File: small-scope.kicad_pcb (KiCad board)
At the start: 2 copper layers, 35.6 x 53.3 mm, 41 parts, among them P1 BNC, P2 AREF, SW1 STAT DIS, U1 LM324N

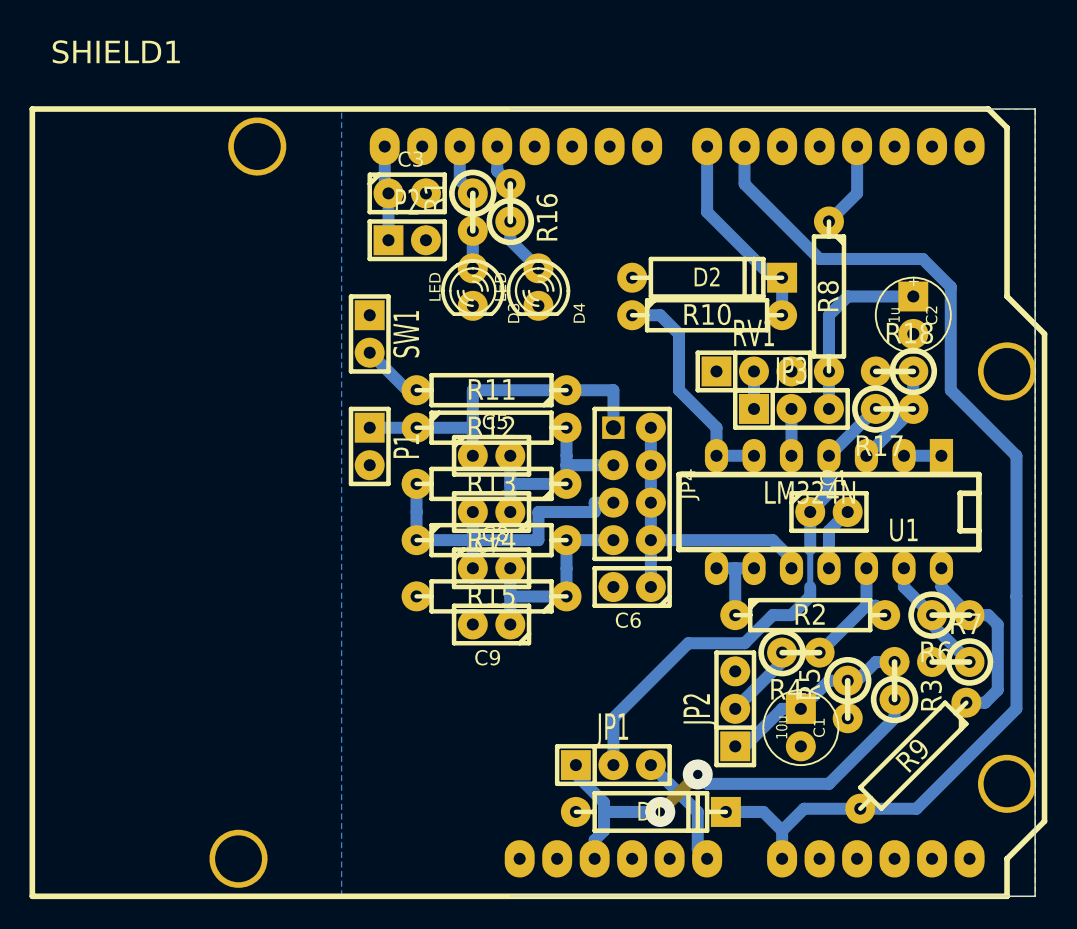
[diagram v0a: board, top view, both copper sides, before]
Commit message: routing done
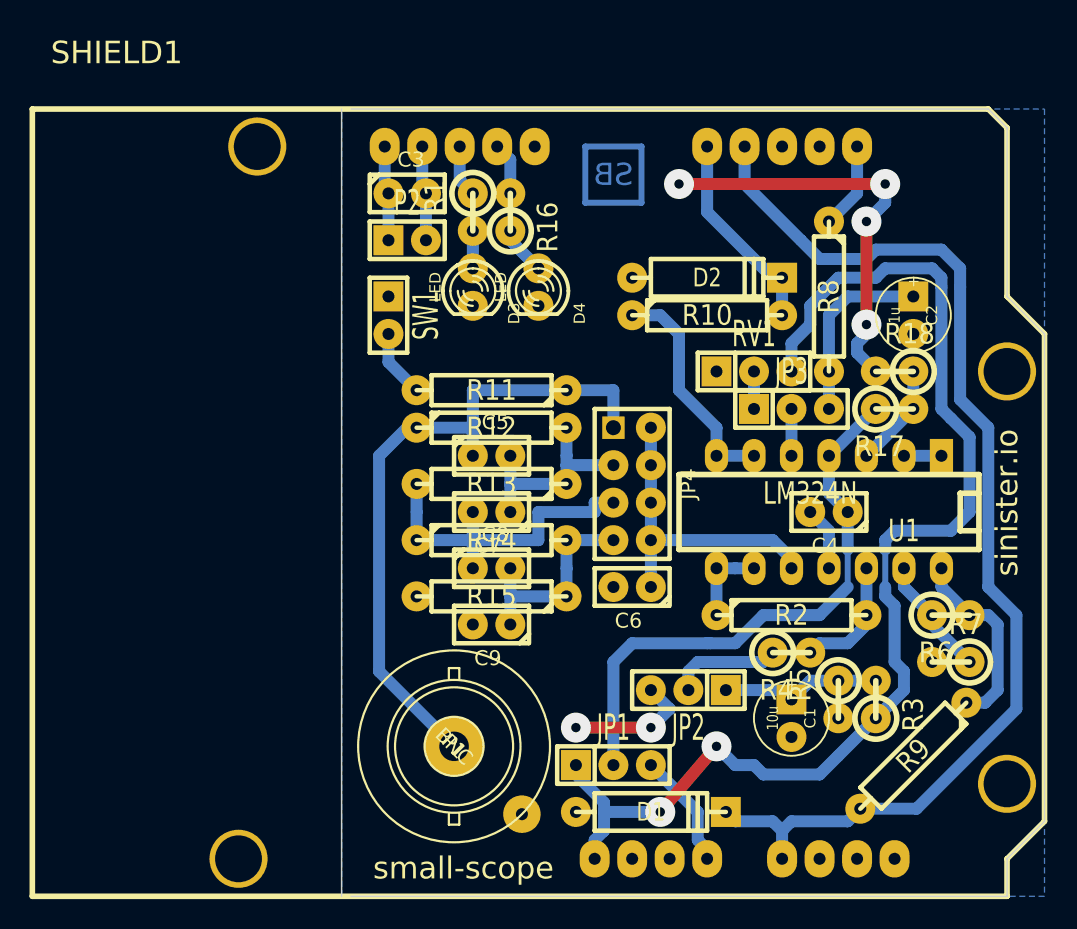
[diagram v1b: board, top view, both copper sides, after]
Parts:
- P1: footprint SIL-2 -> BNCv
- moved P1 21.1 mm to (99.1, 88.3), turned to 135 degrees
- moved JP2 3.42 mm to (114.9, 84.5), turned to 180 degrees
- moved R3 1.80 mm to (127.6, 85.1)
- moved SW1 1.80 mm to (94.6, 59.1)
- moved R2 1.27 mm to (121.9, 79.4)
- moved C1 0.90 mm to (121.9, 86.4)
- moved R4 0.64 mm to (121.9, 81.9)
- moved R5 0.64 mm to (125.1, 85.1)
- moved R16 0.63 mm to (102.9, 52.1)
- turned C4 to 180 degrees
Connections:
- SHIELD1 pad GND1: GND -> (no net)
- SHIELD1 pad GND2: GND -> (no net)
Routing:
- net VCC: track 31.5 -> 82.0 mm
- net GND: track 4.34 -> 47.4 mm, vias 0 -> 6
- net /SIG_IN: track 23.5 -> 45.4 mm
- net (no net): track 0.00 -> 15.2 mm
- net VDD: track 34.5 -> 38.9 mm
- net N-000001: track 5.13 -> 7.51 mm
- net /2.5V: track 13.2 -> 10.9 mm
- net /SIG_UC: track 75.4 -> 77.0 mm
- net N-0000019: track 3.96 -> 3.33 mm
- net /INFO_LED: track 2.91 -> 3.54 mm
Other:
- board size 35.6 x 53.3 mm -> 47.6 x 53.3 mm
- board text added: "SB"
- board text added: "sinister.io"
- board text added: "small-scope"
